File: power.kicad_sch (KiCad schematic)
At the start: 2 parts, among them J3 USB_C_Slave, U1 TPS65987DDHRSHR

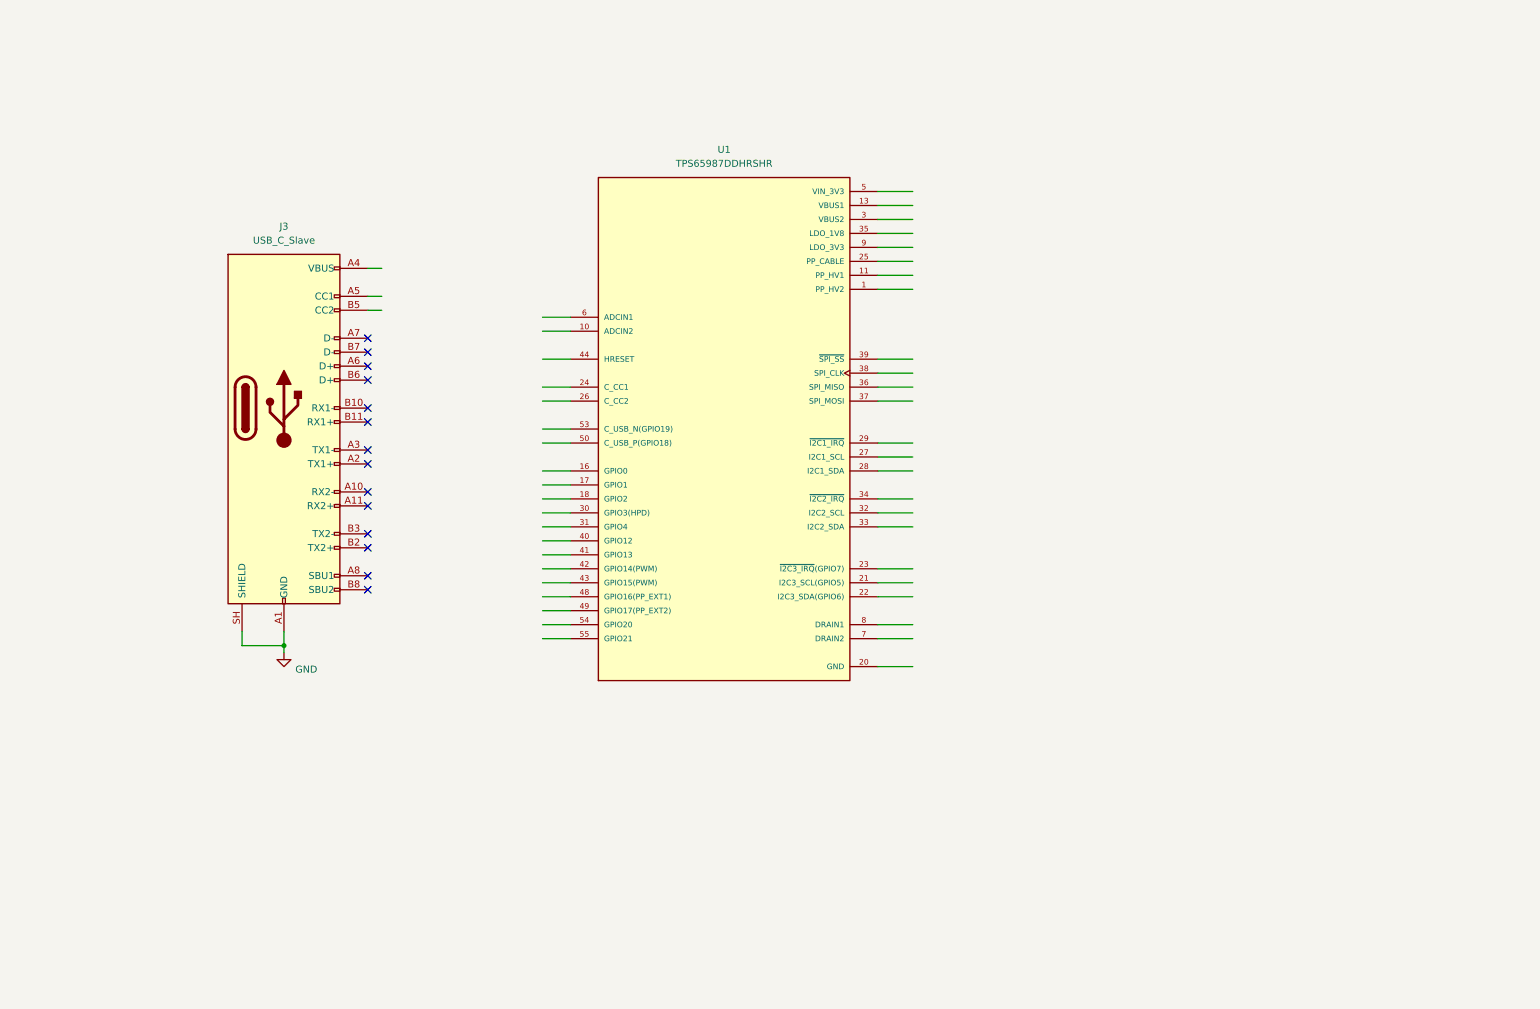
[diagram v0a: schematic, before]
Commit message: Add files via upload
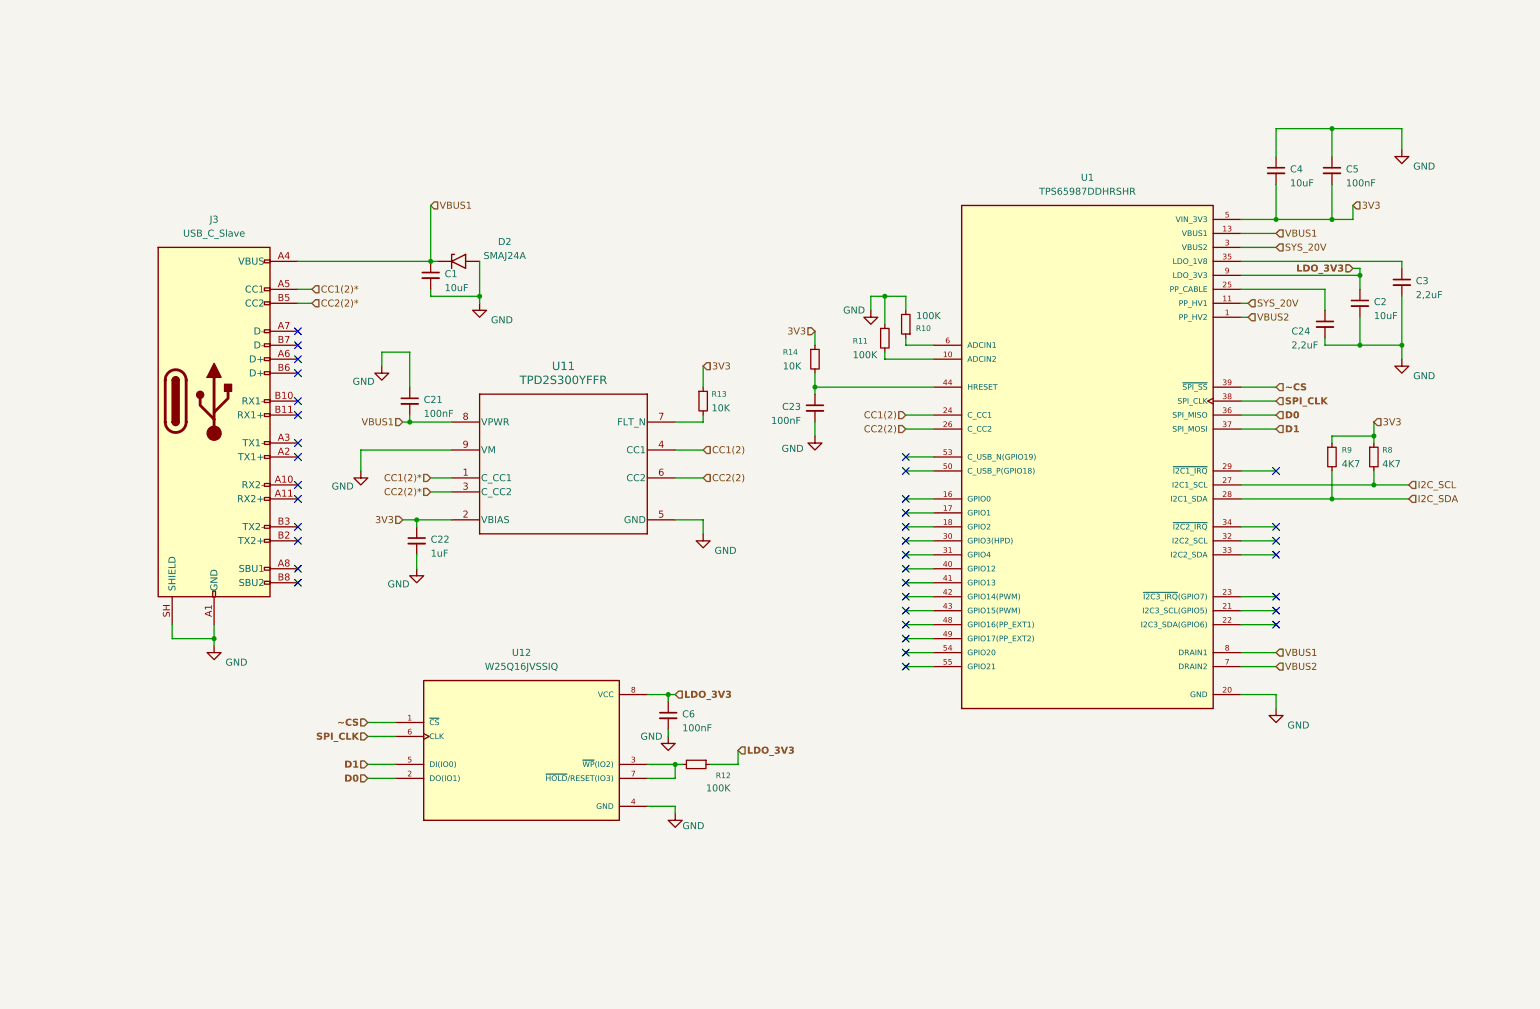
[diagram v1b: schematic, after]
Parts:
- added C1, C2, C4: 10uF, symbol Device:C_Small
- added C21, C23, C5, C6: 100nF, symbol Device:C_Small
- added C22: 1uF, symbol Device:C_Small
- added C24, C3: 2,2uF, symbol Device:C_Small
- added D2: SMAJ24A, Diode_SMD:D_SMA, symbol Diode:SMAJ24A
- added R10, R11, R12: 100K, symbol Device:R_Small
- added R13, R14: 10K, symbol Device:R_Small
- added R8, R9: 4K7, symbol Device:R_Small
- added U11: TPD2S300YFFR, YFF0009AJAJ, symbol TPD2S300YFFR:TPD2S300YFFR
- added U12: W25Q16JVSSIQ, W25Q16JVSSIQ:SOIC127P790X216-8N, symbol W25Q16JVSSIQ:W25Q16JVSSIQ
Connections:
- net GND: now also C1.2, C2.2, C21.1, C22.2, C23.2, C24.2, C3.2, C4.1, C5.1, C6.2, D2.2 (A2), R10.2, R11.1, U11.5 (GND), U11.9 (VM), U12.4 (GND)
- net VBUS2: now reaches U1.1 (PP_HV2)
- net VBUS2: now also U1.52 (DRAIN2), U1.56 (DRAIN2), U1.57 (DRAIN2), U1.57_1 (DRAIN2), U1.57_2 (DRAIN2), U1.57_3 (DRAIN2), U1.57_4 (DRAIN2), U1.57_5 (DRAIN2), U1.57_6 (DRAIN2), U1.7 (DRAIN2)
- net at U1.10 (ADCIN2): now also R11.2
- net SYS_20V: now reaches U1.11 (PP_HV1)
- net SYS_20V: now also U1.3 (VBUS2)
- net VBUS1: now reaches U1.13 (VBUS1)
- net VBUS1: now also J3.A4 (VBUS), J3.A9 (VBUS), J3.B4 (VBUS), J3.B9 (VBUS), U1.15 (DRAIN1), U1.19 (DRAIN1), U1.58 (DRAIN1), U1.58_1 (DRAIN1), U1.58_2 (DRAIN1), U1.58_3 (DRAIN1), U1.58_4 (DRAIN1), U1.58_5 (DRAIN1), U1.58_6 (DRAIN1), U1.8 (DRAIN1), C1.1, C21.2, D2.1 (A1), U11.8 (VPWR)
- net CC1(2): now reaches U1.24 (C_CC1)
- net CC1(2): now also U11.4 (CC1)
- net at U1.25 (PP_CABLE): now also C24.1
- net CC2(2): now reaches U1.26 (C_CC2)
- net CC2(2): now also U11.6 (CC2)
- net I2C_SCL: now reaches U1.27 (I2C1_SCL)
- net I2C_SCL: now also R8.2
- net I2C_SDA: now reaches U1.28 (I2C1_SDA)
- net I2C_SDA: now also R9.2
- net at U1.35 (LDO_1V8): now also C3.1
- net D0: now reaches U1.36 (SPI_MISO)
- net D0: now also U12.2 (DO(IO1))
- net D1: now reaches U1.37 (SPI_MOSI)
- net D1: now also U12.5 (DI(IO0))
- net SPI_CLK: now reaches U1.38 (SPI_CLK)
- net SPI_CLK: now also U12.6 (CLK)
- net ~CS: now reaches U1.39 (~{SPI_SS})
- net ~CS: now also U12.1 (~{CS})
- net at U1.44 (HRESET): now also C23.1, R14.2
- net 3V3: now reaches U1.5 (VIN_3V3)
- net 3V3: now also C22.1, C4.2, C5.2, R13.1, R14.1, R8.1, R9.1, U11.2 (VBIAS)
- net at U1.6 (ADCIN1): now also R10.1
- net LDO_3V3: now reaches U1.9 (LDO_3V3)
- net LDO_3V3: now also C2.1, C6.1, R12.1, U12.8 (VCC)
- net CC1(2)*: now reaches J3.A5 (CC1)
- net CC1(2)*: now also U11.1 (C_CC1)
- net CC2(2)*: now reaches J3.B5 (CC2)
- net CC2(2)*: now also U11.3 (C_CC2)
- new net: R12.2, U12.3 (~{WP}(IO2)), U12.7 (~{HOLD}/RESET(IO3))
- new net: R13.2, U11.7 (FLT_N)
- no-connect marks 14 -> 36
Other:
- moved on the sheet: J3, U1

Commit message: Add files via upload
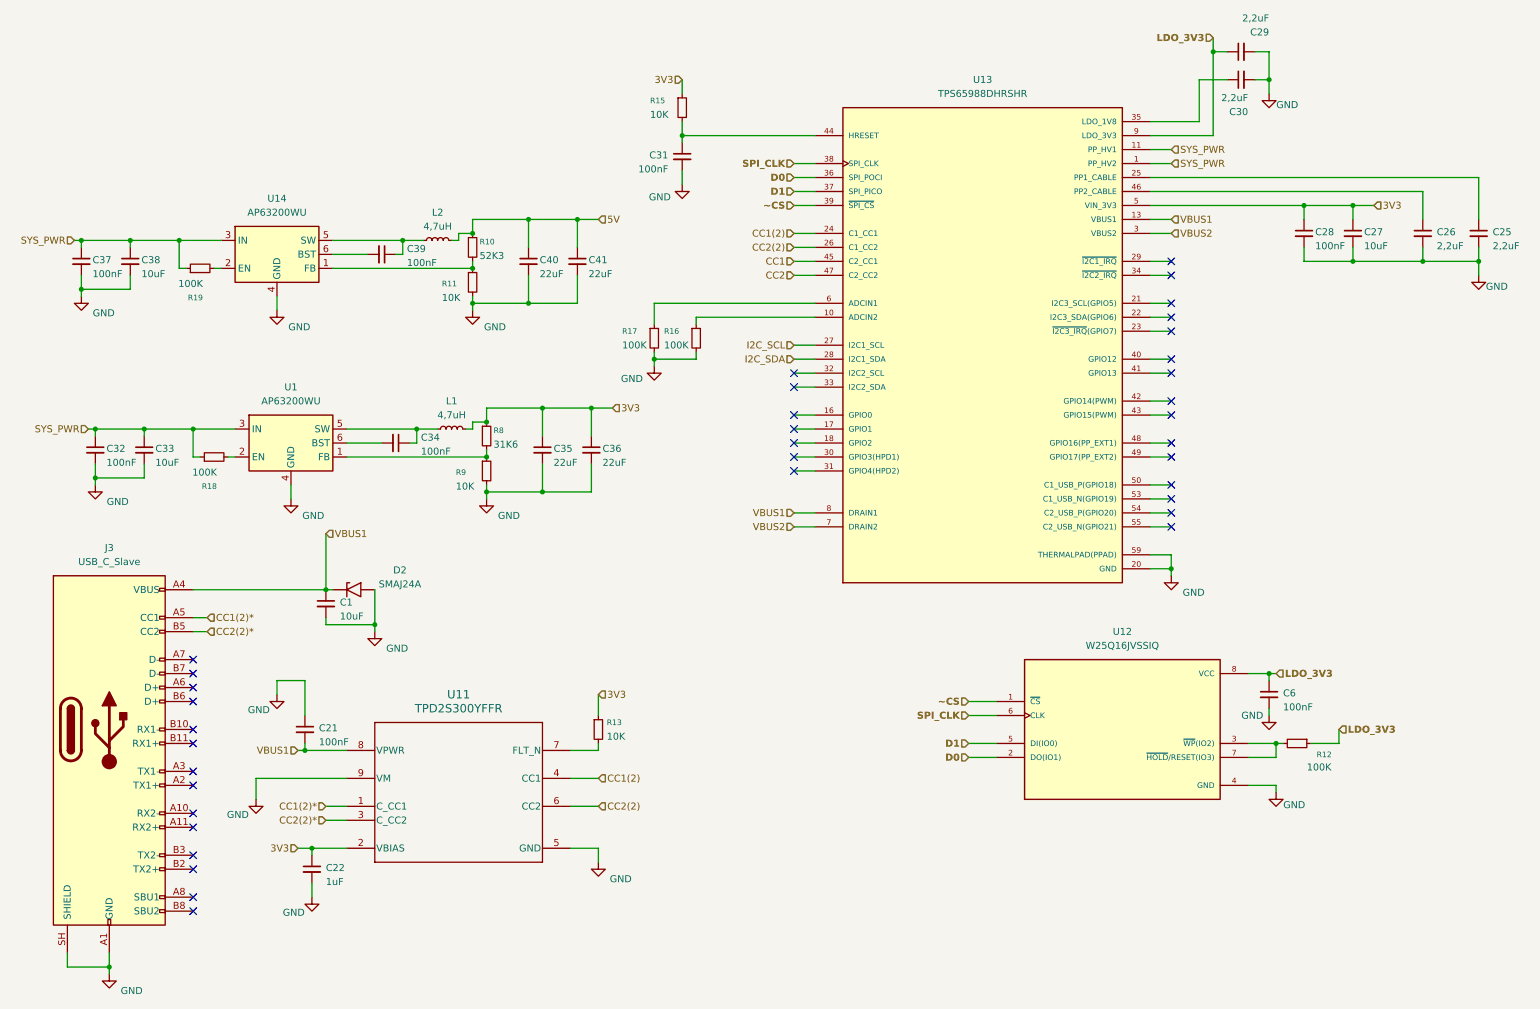
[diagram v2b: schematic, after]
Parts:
- removed C2, C4: 10uF, symbol Device:C_Small
- removed C23, C5: 100nF, symbol Device:C_Small
- removed C24, C3: 2,2uF, symbol Device:C_Small
- removed R14: 10K, symbol Device:R_Small
- removed U1: TPS65987DDHRSHR, TPS65987DDHRSHR:IC_TPS65987DDHRSHR, symbol TPS65987DDHRSHR:TPS65987DDHRSHR
- added C25, C26, C29, C30: 2,2uF, symbol Device:C_Small
- added C27, C33, C38: 10uF, symbol Device:C_Small
- added C28, C31, C32, C34, C37, C39: 100nF, symbol Device:C_Small
- added C35, C36, C40, C41: 22uF, symbol Device:C_Small
- added L1, L2: 4,7uH, symbol Device:L_Small
- added R15: 10K, symbol Device:R_Small
- added R16, R17, R18, R19: 100K, symbol Device:R_Small
- added U1, U14: AP63200WU, Package_TO_SOT_SMD:TSOT-23-6, symbol Regulator_Switching:AP63200WU
- added U13: TPS65988DHRSHR, TPS65988DHRSHR:IC_TPS65987DDHRSHR, symbol TPS65988DHRSHR:TPS65988DHRSHR
- R10: value 100K -> 52K3
- R11: value 100K -> 10K
- R8: value 4K7 -> 31K6
- R9: value 4K7 -> 10K
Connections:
- net 3V3: now also C27.1, C28.1, C35.1, C36.1, L1.2, R15.1, U13.5 (VIN_3V3); no longer R9.1
- net CC1(2): now also U13.24 (C1_CC1)
- net CC2(2): now also U13.26 (C1_CC2)
- net D0: now also U13.36 (SPI_POCI)
- net D1: now also U13.37 (SPI_PICO)
- net GND: now also R11.2, R9.2, C25.2, C26.2, C27.2, C28.2, C29.2, C30.2, C31.2, C32.2, C33.2, C35.2, C36.2, C37.2, C38.2, C40.2, C41.2, R16.2, R17.2, U1.4 (GND), U13.20 (GND), U13.51 (GND), U13.59 (THERMALPAD(PPAD)), U14.4 (GND); no longer R10.2, R11.1
- net I2C_SCL: now also U13.27 (I2C1_SCL); no longer R8.2
- net I2C_SDA: now also U13.28 (I2C1_SDA); no longer R9.2
- net LDO_3V3: now also C29.1, U13.9 (LDO_3V3)
- net SPI_CLK: now also U13.38 (SPI_CLK)
- net VBUS1: now also U13.13 (VBUS1), U13.15 (DRAIN1), U13.19 (DRAIN1), U13.58 (DRAIN1), U13.8 (DRAIN1)
- net VBUS2: now also U13.3 (VBUS2), U13.52 (DRAIN2), U13.56 (DRAIN2), U13.57 (DRAIN2), U13.7 (DRAIN2)
- net ~CS: now also U13.39 (~{SPI_CS})
- net 5V: now reaches R10.1
- net 5V: now also C40.1, C41.1, L2.2
- new net: C39.1, L2.1, U14.5 (SW)
- new net: R10.2, R11.1, U14.1 (FB)
- new net: R8.2, R9.1, U1.1 (FB)
- new net: R18.2, U1.2 (EN)
- new net: C34.1, L1.1, U1.5 (SW)
- new net: C34.2, U1.6 (BST)
- new net: C31.1, R15.2, U13.44 (HRESET)
- new net: R16.1, U13.10 (ADCIN2)
- new net: R17.1, U13.6 (ADCIN1)
- new net: C25.1, U13.25 (PP1_CABLE)
- new net: C30.1, U13.35 (LDO_1V8)
- new net: C26.1, U13.46 (PP2_CABLE)
- new net: R19.2, U14.2 (EN)
- new net: C39.2, U14.6 (BST)
- new net CC1: U13.45 (C2_CC1)
- new net CC2: U13.47 (C2_CC2)
- new net SYS_PWR: C32.1, C33.1, C37.1, C38.1, R18.1, R19.1, U1.3 (IN), U13.1 (PP_HV2), U13.11 (PP_HV1), U14.3 (IN)
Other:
- moved on the sheet: C1, C21, C22, C6, D2, J3, R12, R13, U11, U12
